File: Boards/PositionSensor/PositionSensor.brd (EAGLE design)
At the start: 17.8 x 27.9 mm, 4 parts

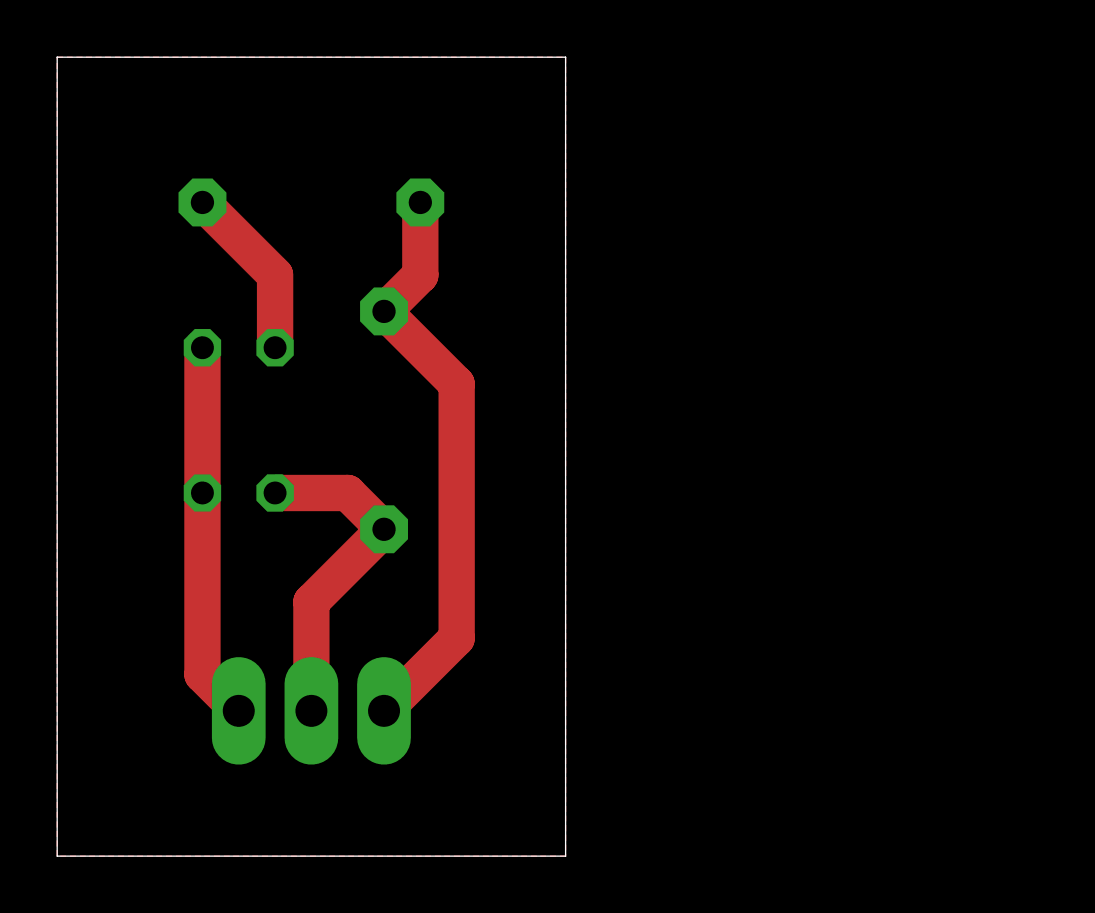
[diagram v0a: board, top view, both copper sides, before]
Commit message: finished for mass production
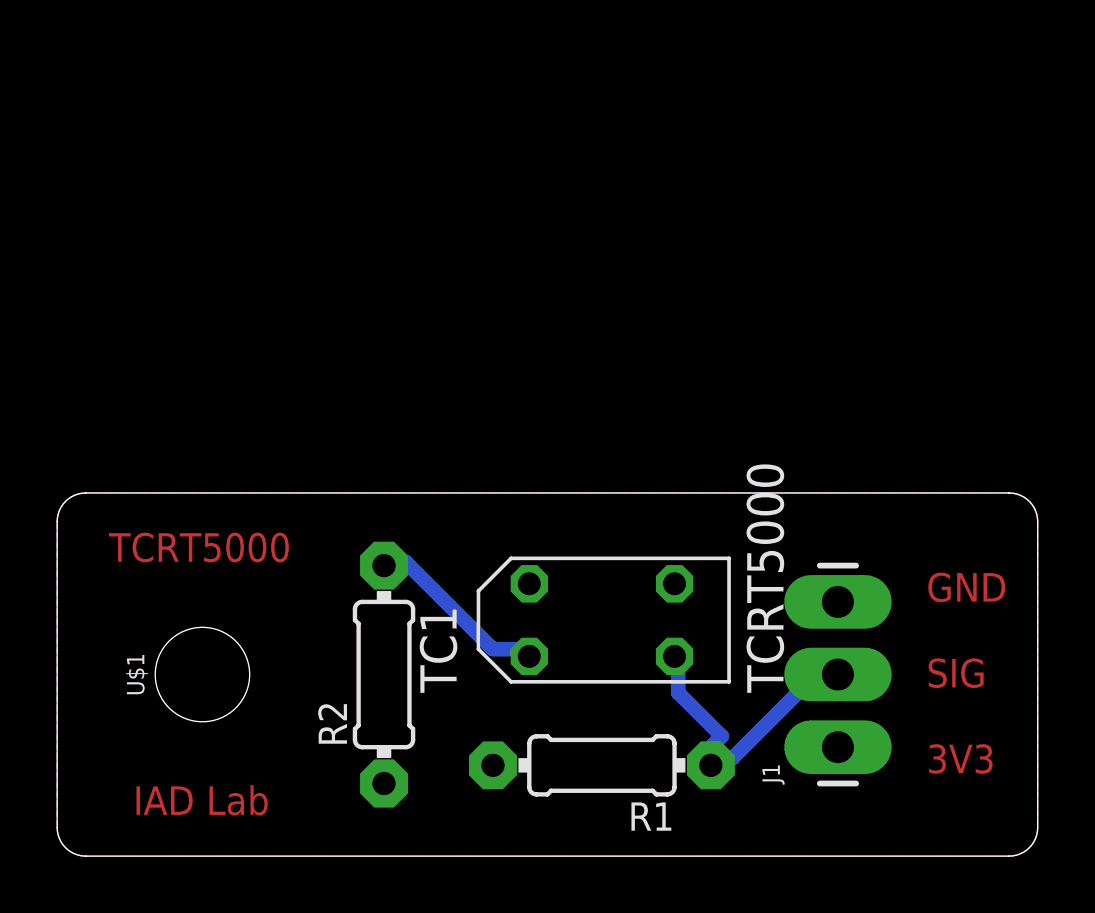
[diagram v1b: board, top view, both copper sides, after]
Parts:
- added U$1: (no value), SparkFun-Hardware:STAND-OFF
- moved R2 16.7 mm to (11.4, 6.35), flipped to the top, turned to 90 degrees
- moved J1 15.9 mm to (27.3, 3.81), flipped to the top, turned to 90 degrees
- moved TC1 14.5 mm to (19.1, 8.26), flipped to the top, turned to 90 degrees
- moved R1 14.3 mm to (19.1, 3.17), flipped to the top, turned to 180 degrees
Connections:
- net VCC renamed 3V3
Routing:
- net 3V3: track 20.4 -> 0.00 mm
- net GND: track 13.2 -> 0.00 mm
- net SIG: track 11.7 -> 11.1 mm
- added copper zone on layer 1, net 3V3
- added copper zone on layer 16, net GND
- removed copper zone on layer 1, net N$2
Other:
- board size 17.8 x 27.9 mm -> 34.3 x 12.7 mm
- board text added: "GND SIG 3V3"
- board text added: "IAD Lab"
- board text added: "TCRT5000"
